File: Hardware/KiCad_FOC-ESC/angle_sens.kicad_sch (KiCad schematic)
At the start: 2 parts, among them IC6 MA702GQ-P, U3 MT6701CT

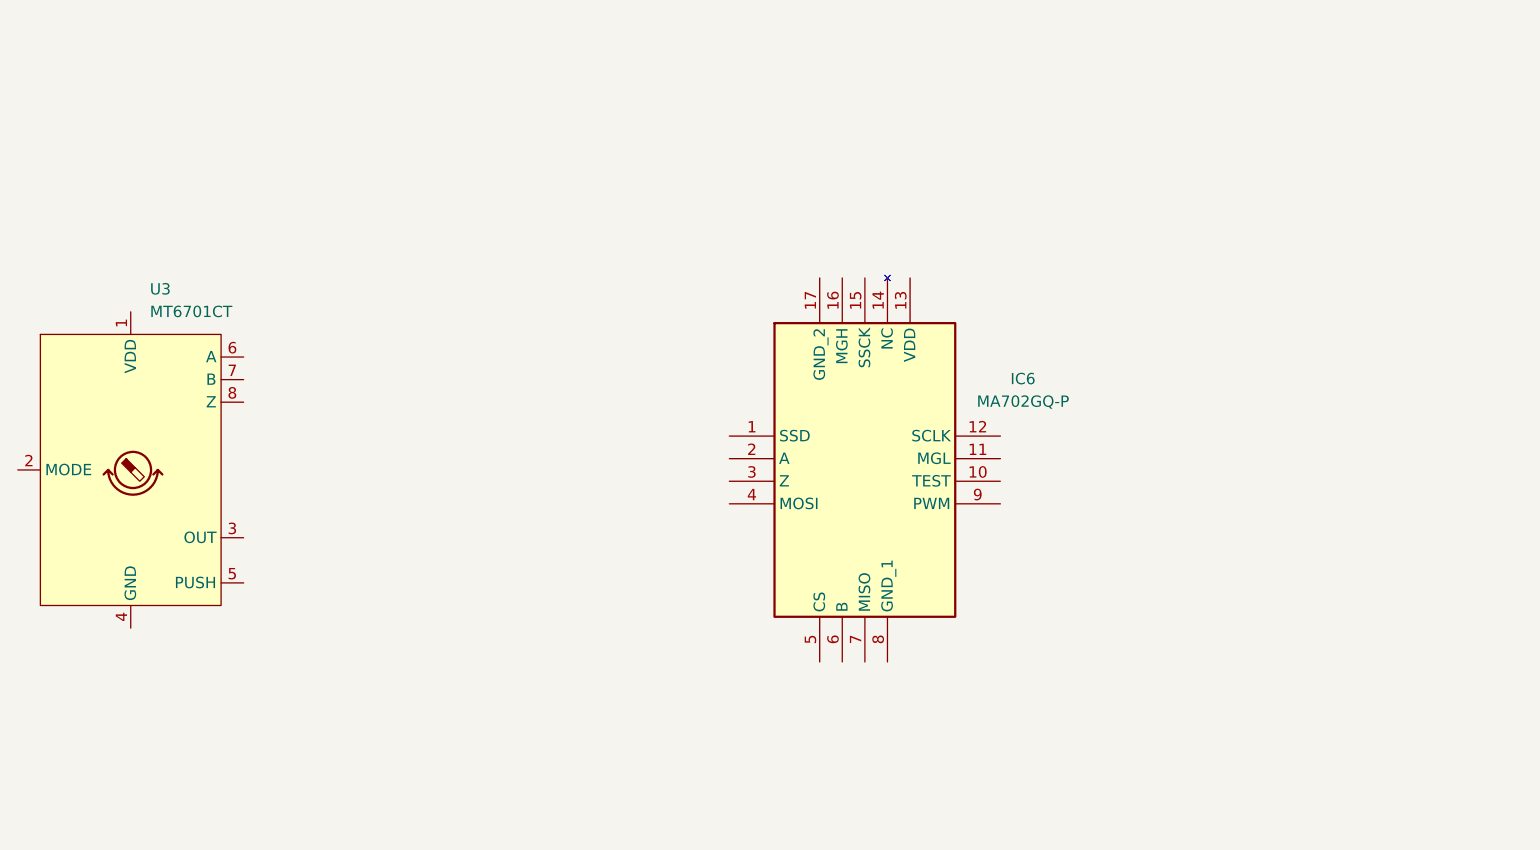
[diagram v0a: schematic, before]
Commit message: added:ferrite bead
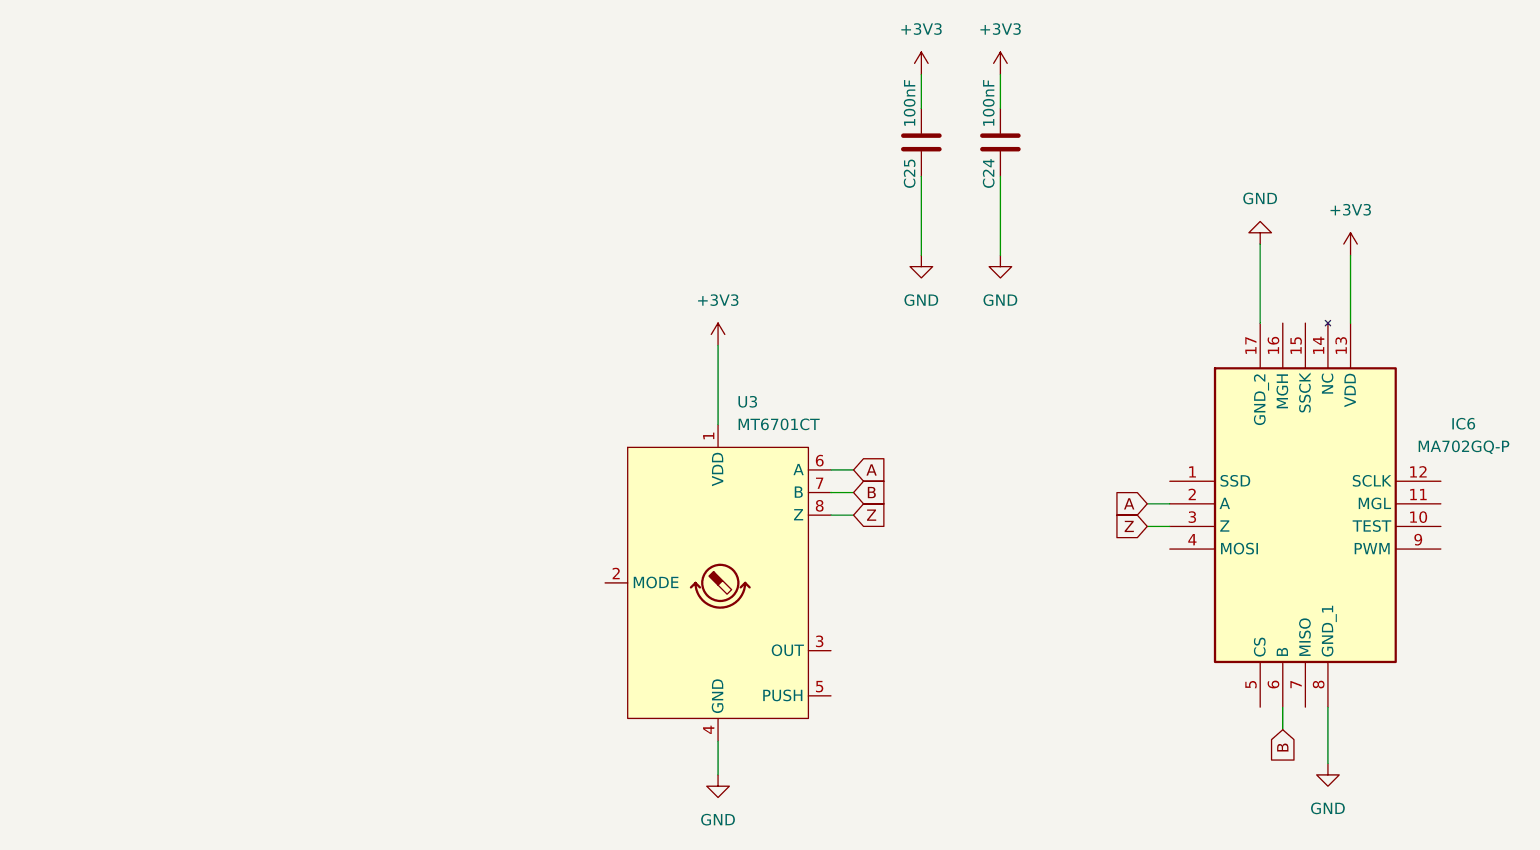
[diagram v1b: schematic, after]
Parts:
- added C24, C25: 100nF, Capacitor_SMD:C_0402_1005Metric, symbol Device:C
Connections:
- net +3V3: now reaches U3.1 (VDD)
- net +3V3: now also IC6.13 (VDD), C24.2, C25.2
- net GND: now reaches U3.4 (GND)
- net GND: now also IC6.17 (GND_2), IC6.8 (GND_1), C24.1, C25.1
- net A: now reaches U3.6 (A)
- net A: now also IC6.2 (A)
- net B: now reaches U3.7 (B)
- net B: now also IC6.6 (B)
- net Z: now reaches U3.8 (Z)
- net Z: now also IC6.3 (Z)
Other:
- moved on the sheet: IC6, U3
